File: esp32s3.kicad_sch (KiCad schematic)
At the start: 40 parts, among them J1 Conn_01x05, U5 ESP32-S3R8, U6 W25Q128JVSIQ, U7 MPR121QR2, Y1 40MHz

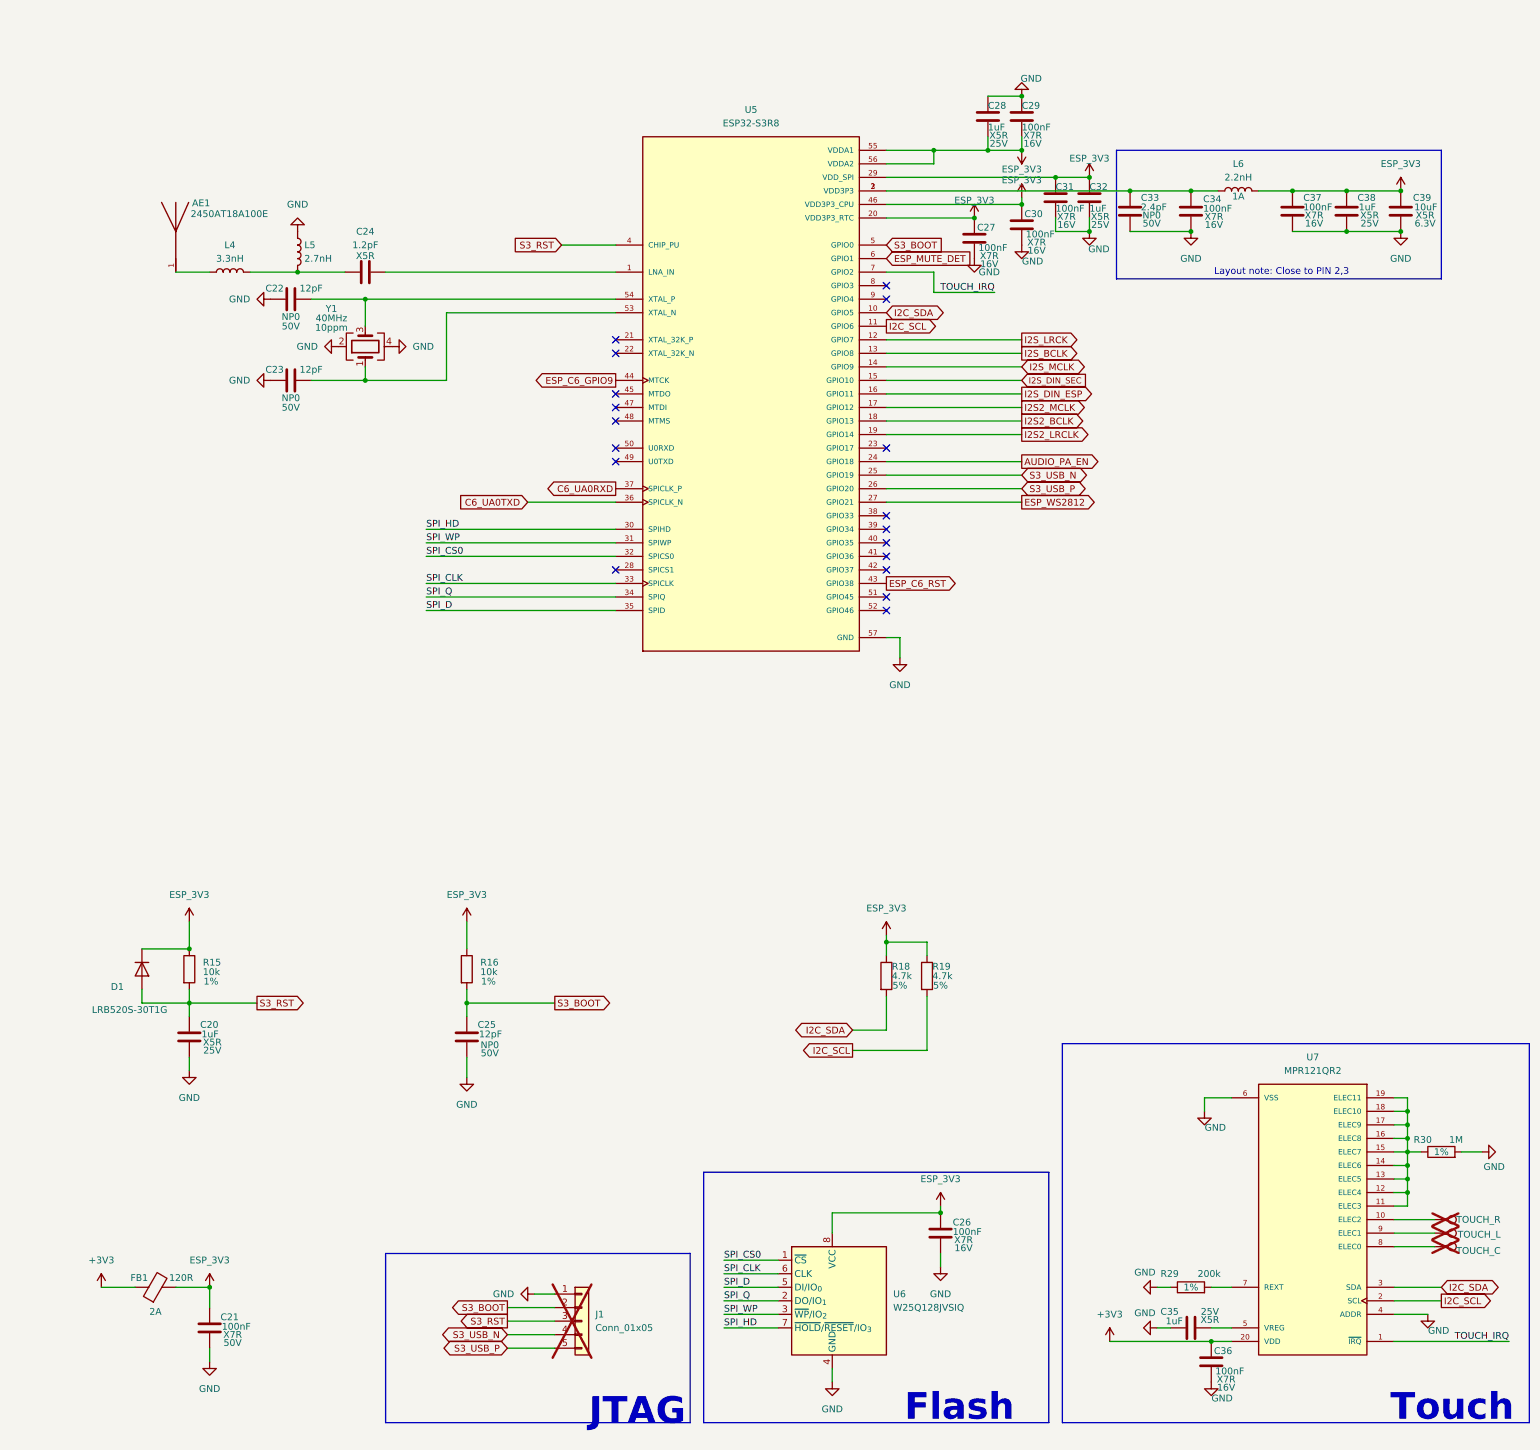
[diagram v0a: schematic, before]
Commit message: v3 hardware changes
Full redesing, ready for prototype order
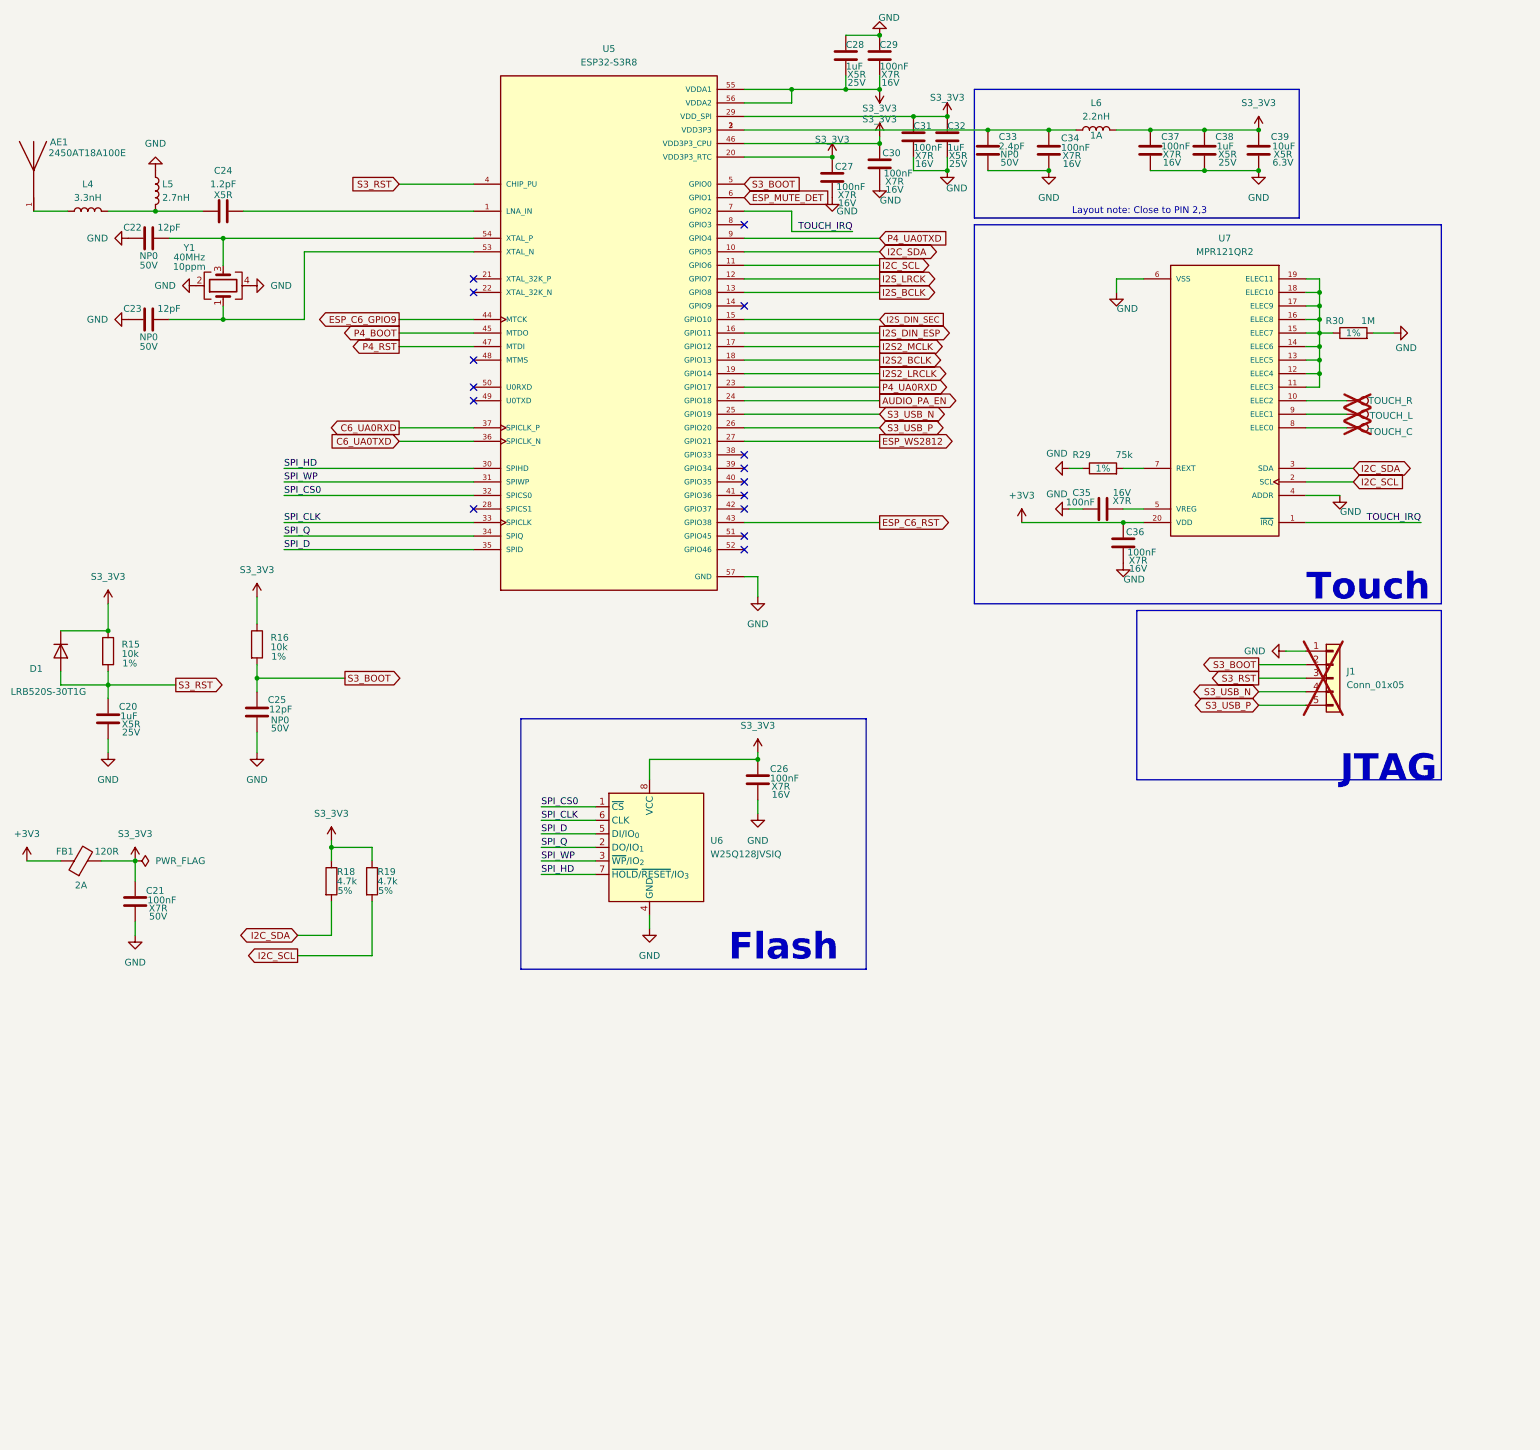
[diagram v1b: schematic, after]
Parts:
- C35: value 1uF -> 100nF; Dielectric X5R -> X7R; LCSC Part # C52923 -> (none); MPN CL05A105KA5NQNC -> CL05B104KO5NNNC; Manufacturer Part CL05A105KA5NQNC -> (none); Voltage 25V -> 16V
- R29: value 200k -> 75k; LCSC Part # C25764 -> (none); MPN 0402WGF2003TCE -> 0402WGF7502TCE
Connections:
- net P4_UA0RXD: now reaches U5.23 (GPIO17)
- net P4_BOOT: now reaches U5.45 (MTDO)
- net P4_RST: now reaches U5.47 (MTDI)
- net P4_UA0TXD: now reaches U5.9 (GPIO4)
- net ESP_3V3 renamed S3_3V3
- net I2S_MCLK: no longer names the net of U5.14 (GPIO9)
- no-connect marks 18 -> 15
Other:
- moved on the sheet: AE1, C20, C21, C22, C23, C24, C25, C26, C27, C28, C29, C30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
